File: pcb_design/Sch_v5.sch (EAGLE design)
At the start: 32 parts

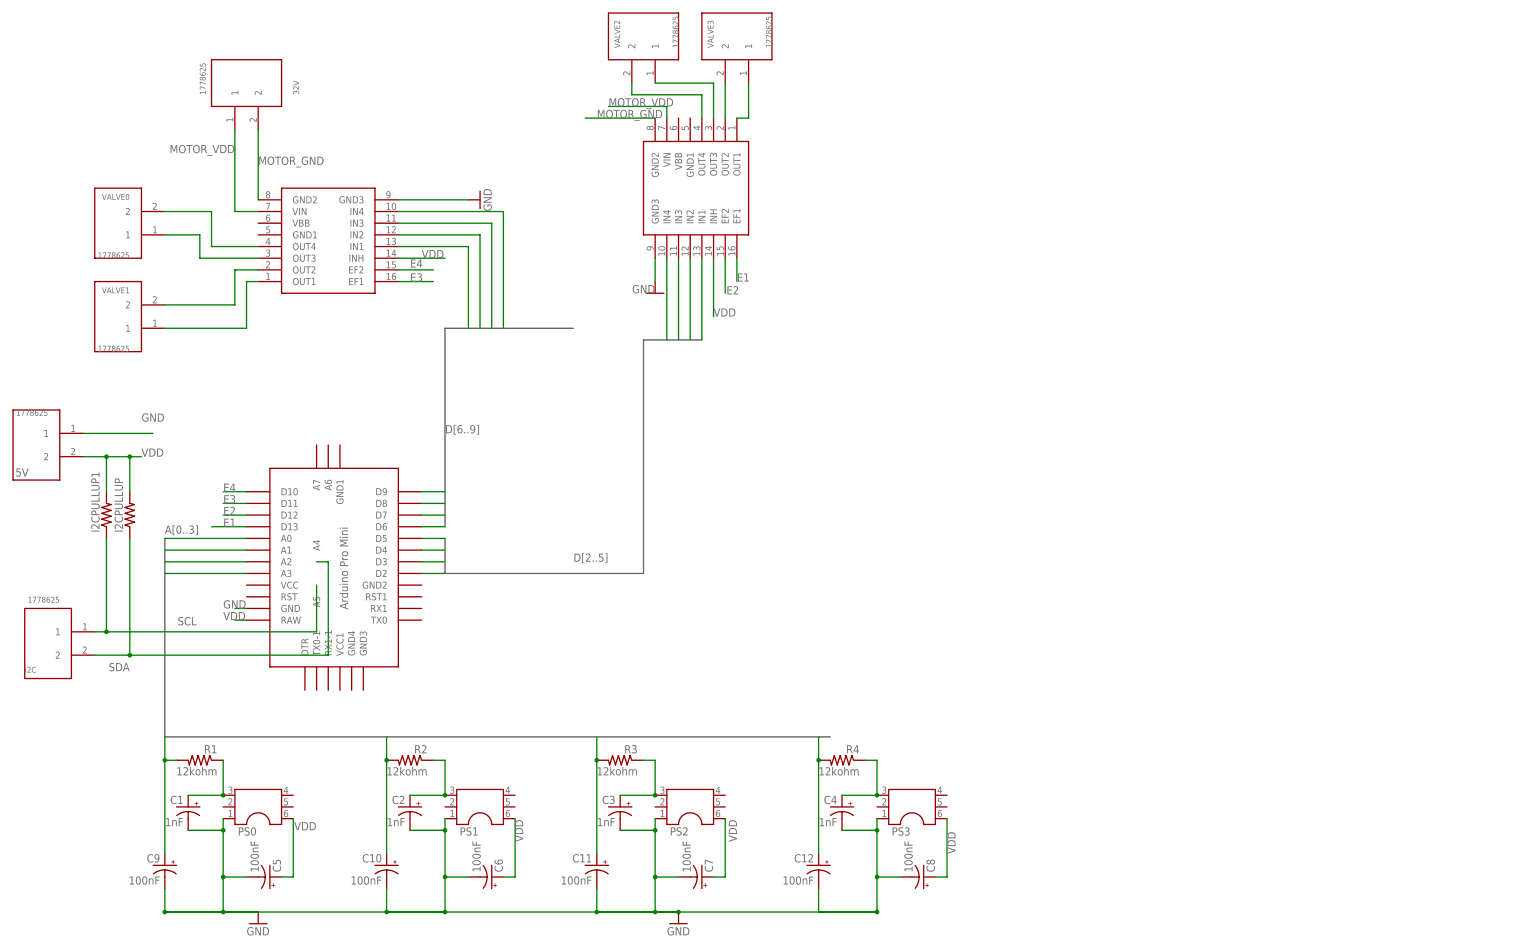
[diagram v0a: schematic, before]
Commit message: commiting recent work
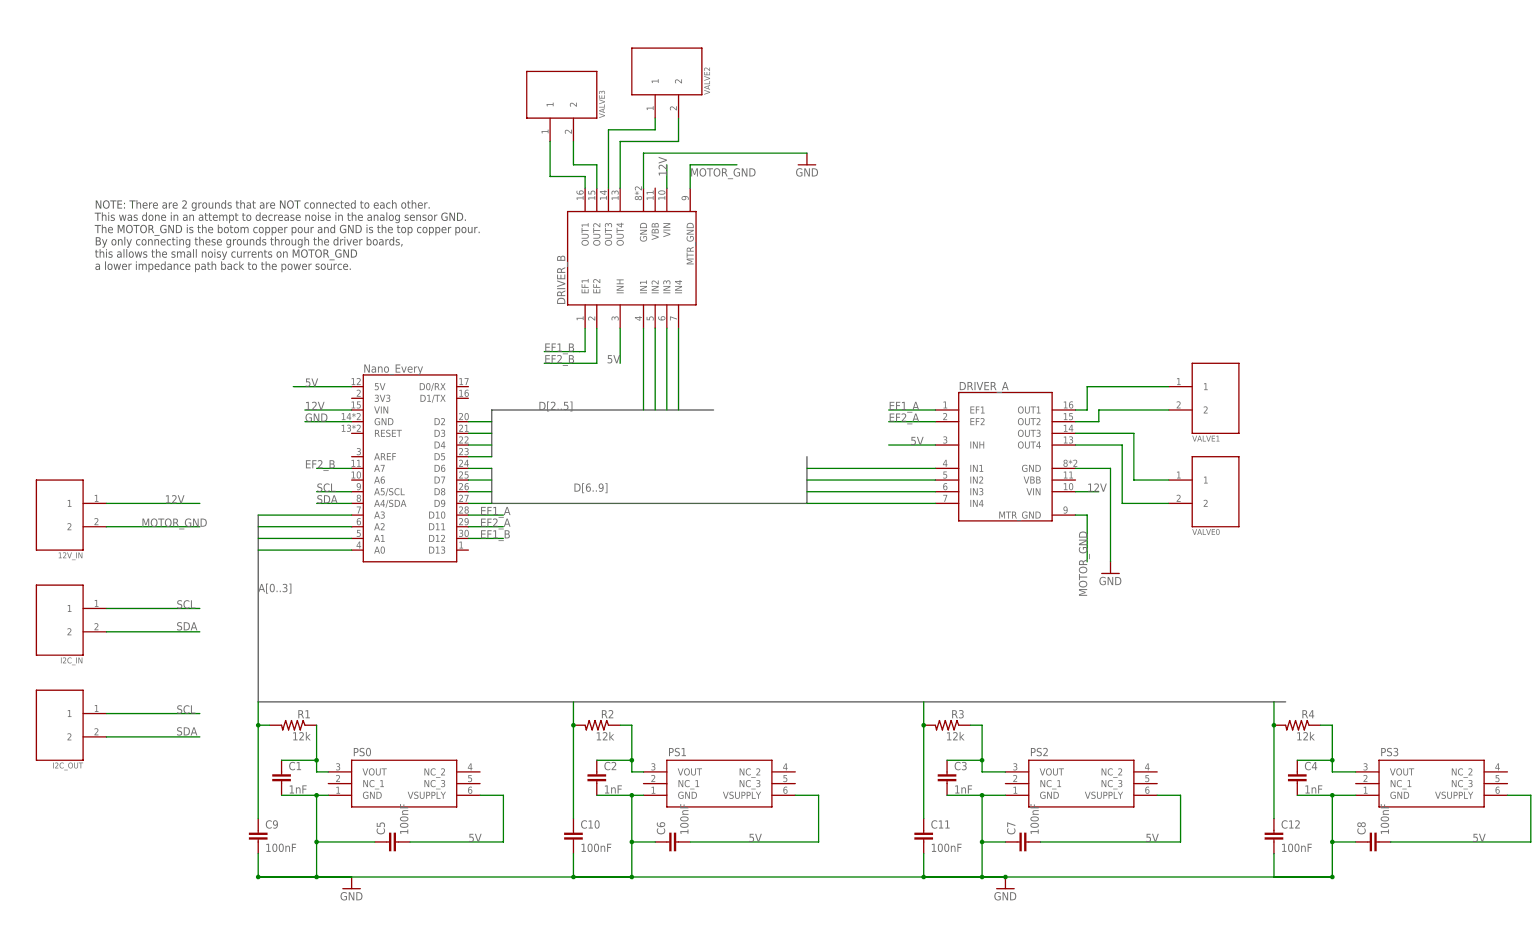
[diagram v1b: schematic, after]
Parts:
- removed 32V, 5V, I2C: 1778625, 1778625:1778625
- removed I2CPULLUP, I2CPULLUP1: (no value), rcl:R-US_0204/7
- removed U$1: ABK-PRO-MINI, Arduino-clone:ABK-PRO-MINI
- removed U$2, U$3: A4990, pololu-stepper-driver:A4990
- added 12V_IN, I2C_IN, I2C_OUT: PHOENIX_CONNECTOR_1778625, byu_pressure_control:PHOENIX_CONNECTOR_1778625
- added DRIVER_A, DRIVER_B: A4990_DUAL_MOTOR_DRIVER_CARRIER, byu_pressure_control:A4990_DUAL_MOTOR_DRIVER_CARRIER
- added NANO: ARDUINO_NANO_EVERY, byu_pressure_control:ARDUINO_NANO_EVERY
- C1, C10, C11, C12, C2, C3, C4, C5, C6, C7, C8, C9: device rcl:CPOL-USE2.5-5 -> byu_pressure_control:CERAMIC_CAPACITOR
- PS0, PS1, PS2, PS3: value (none) -> PRESSURE_SENSOR_ABPDRNN100PGAA5; device RAD_2:ABPDRNN100PGAA5 -> byu_pressure_control:PRESSURE_SENSOR_ABPDRNN100PGAA5
- R1, R2, R3, R4: value 12kohm -> 12k
- VALVE0, VALVE1, VALVE2, VALVE3: value 1778625 -> PHOENIX_CONNECTOR_1778625; device 1778625:1778625 -> byu_pressure_control:PHOENIX_CONNECTOR_1778625
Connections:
- removed net E1: U$1.D13, U$3.EF1
- removed net E2: U$1.D12, U$3.EF2
- removed net E3: U$1.D11, U$2.EF1
- removed net E4: U$1.D10, U$2.EF2
- removed net MOTOR_VDD: 32V.1, U$2.VIN, U$3.VIN
- removed net N$13: U$3.OUT1, VALVE3.1
- removed net N$14: U$3.OUT2, VALVE3.2
- removed net N$15: U$3.OUT3, VALVE2.1
- removed net N$16: U$3.OUT4, VALVE2.2
- removed net VDD: 5V.2, C5.+, C6.+, C7.+, C8.+, I2CPULLUP.2, I2CPULLUP1.2, PS0.6, PS1.6, PS2.6, PS3.6, U$1.RAW, U$2.INH, U$3.INH
- new net 12V: 12V_IN.1, DRIVER_A.VIN, DRIVER_B.VIN, NANO.VIN
- new net 5V: C5.2, C6.2, C7.2, C8.2, DRIVER_A.INH, DRIVER_B.INH, NANO.5V, PS0.VSUPPLY, PS1.VSUPPLY, PS2.VSUPPLY, PS3.VSUPPLY
- new net EF1_A: DRIVER_A.EF1, NANO.D10
- new net EF1_B: DRIVER_B.EF1, NANO.D12
- new net EF2_A: DRIVER_A.EF2, NANO.D11
- new net EF2_B: DRIVER_B.EF2, NANO.A7
- new net N$10: DRIVER_B.OUT2, VALVE3.2
- new net N$11: DRIVER_B.OUT3, VALVE2.1
- new net N$12: DRIVER_B.OUT4, VALVE2.2
- new net N$9: DRIVER_B.OUT1, VALVE3.1
- net A0: now also C9.1, NANO.A0; no longer C9.+, U$1.A0
- net A1: now also C10.1, NANO.A1; no longer C10.+, U$1.A1
- net A2: now also C11.1, NANO.A2; no longer C11.+, U$1.A2
- net A3: now also C12.1, NANO.A3; no longer C12.+, U$1.A3
- net D2: now also DRIVER_B.IN1, NANO.D2; no longer U$1.D2, U$3.IN1
- net D3: now also DRIVER_B.IN2, NANO.D3; no longer U$1.D3, U$3.IN2
- net D4: now also DRIVER_B.IN3, NANO.D4; no longer U$1.D4, U$3.IN3
- net D5: now also DRIVER_B.IN4, NANO.D5; no longer U$1.D5, U$3.IN4
- net D6: now also DRIVER_A.IN1, NANO.D6; no longer U$1.D6, U$2.IN1
- net D7: now also DRIVER_A.IN2, NANO.D7; no longer U$1.D7, U$2.IN2
- net D8: now also DRIVER_A.IN3, NANO.D8; no longer U$1.D8, U$2.IN3
- net D9: now also DRIVER_A.IN4, NANO.D9; no longer U$1.D9, U$2.IN4
- net GND: now also C1.2, C10.2, C11.2, C12.2, C2.2, C3.2, C4.2, C5.1, C6.1, C7.1, C8.1, C9.2, DRIVER_A.GND, DRIVER_B.GND, NANO.GND, PS0.GND, PS1.GND, PS2.GND, PS3.GND; no longer 5V.1, C1.-, C10.-, C11.-, C12.-, C2.-, C3.-, C4.-, C5.-, C6.-, C7.-, C8.-, C9.-, PS0.1, PS1.1, PS2.1, PS3.1, U$1.GND, U$2.GND3, U$3.GND3
- net MOTOR_GND: now also 12V_IN.2, DRIVER_A.MTR_GND, DRIVER_B.MTR_GND; no longer 32V.2, U$2.GND2, U$3.GND2
- net N$1: now also C1.1, PS0.VOUT; no longer C1.+, PS0.3
- net N$2: now also C2.1, PS1.VOUT; no longer C2.+, PS1.3
- net N$3: now also C3.1, PS2.VOUT; no longer C3.+, PS2.3
- net N$4: now also C4.1, PS3.VOUT; no longer C4.+, PS3.3
- net N$5: now also DRIVER_A.OUT2; no longer U$2.OUT2
- net N$6: now also DRIVER_A.OUT1; no longer U$2.OUT1
- net N$7: now also DRIVER_A.OUT3; no longer U$2.OUT3
- net N$8: now also DRIVER_A.OUT4; no longer U$2.OUT4
- net SCL: now also I2C_IN.1, I2C_OUT.1, NANO.A5/SCL; no longer I2C.1, I2CPULLUP1.1, U$1.A5
- net SDA: now also I2C_IN.2, I2C_OUT.2, NANO.A4/SDA; no longer I2C.2, I2CPULLUP.1, U$1.A4
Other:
- note added: "NOTE: There are 2 grounds that are NOT connected to each other. This was done in an attempt to decrease noise in the analog sensor GND. The MOTOR_GND is the botom copper pour and GND is the top copper pour. By only connecting these grounds through the driver boards, this allows the small noisy currents on MOTOR_GND a lower impedance path back to the power source."
- note removed: "5V"
- moved on the sheet: R1, R2, R3, R4, VALVE0, VALVE1, VALVE2, VALVE3
